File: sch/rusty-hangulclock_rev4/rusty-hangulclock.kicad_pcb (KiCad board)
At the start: 2 copper layers, 170 x 170 mm, 90 parts, among them J1 Conn_OLED, J2 Conn_OLED, J3 Conn_USB2, J4 USB_C_Receptacle_PowerOnly_6P, Q1 S8050, SW1 RotaryEncoder_Switch_MP, U1 ESP32-C3-WROOM-02, U2 SY8088, U3 DS3231MZ

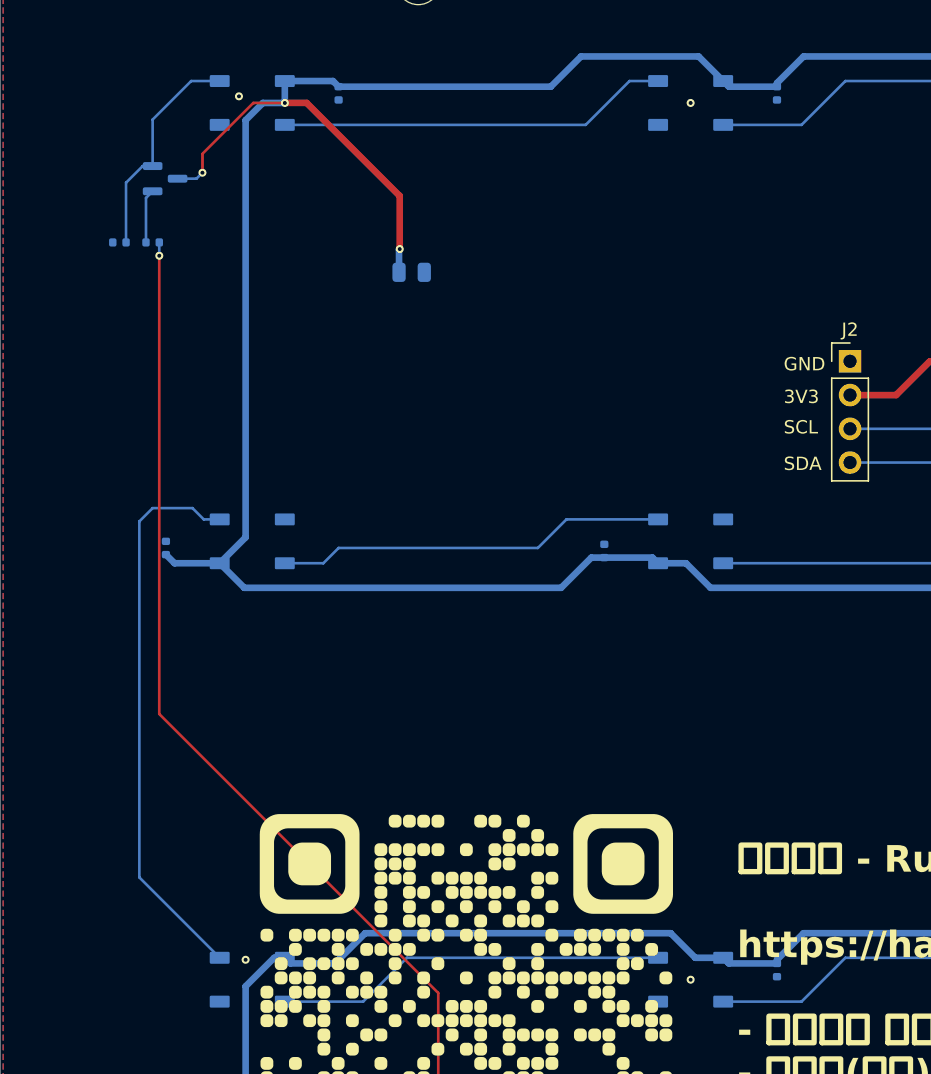
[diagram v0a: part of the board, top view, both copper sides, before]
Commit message: fix: sch
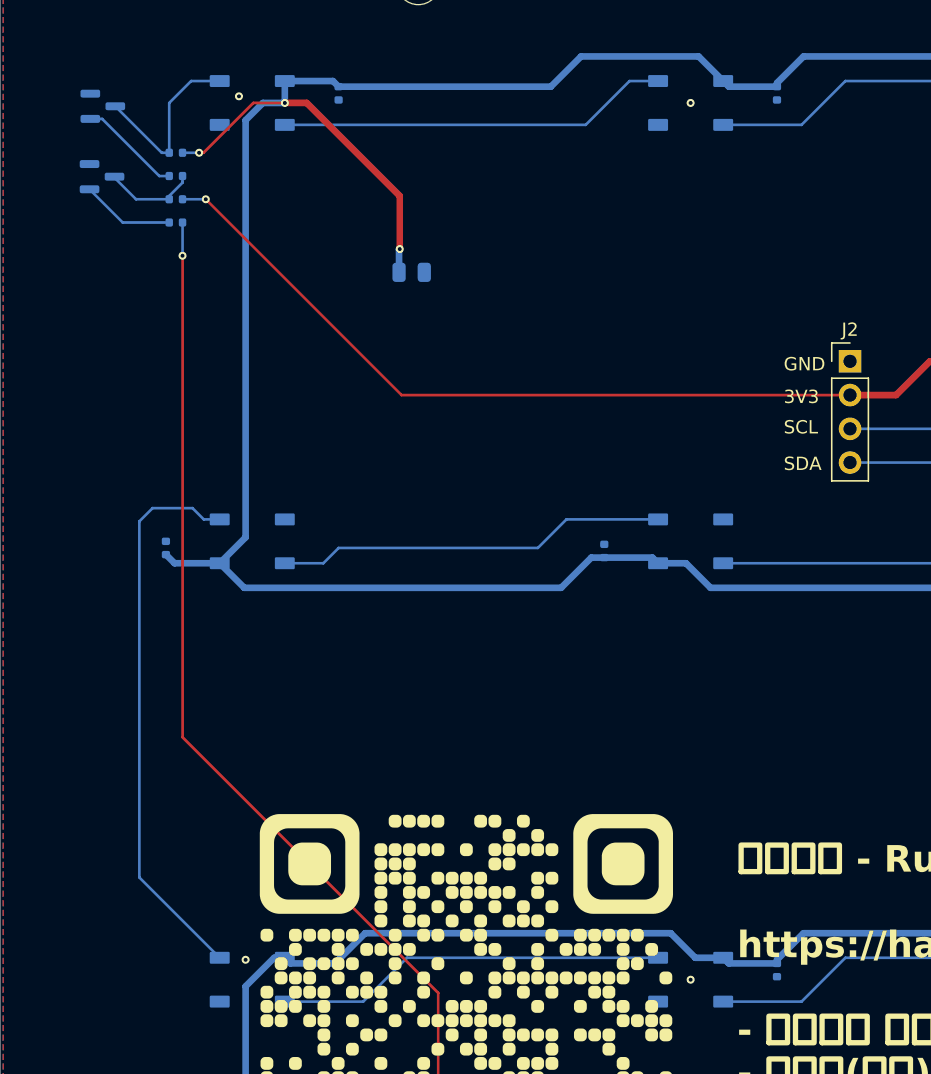
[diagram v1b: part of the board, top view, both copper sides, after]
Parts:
- removed R9: 10kΩ, PCM_JLCPCB:R_0402
- added Q2: S8050, PCM_JLCPCB:Q_SOT-23, B.Cu at (30.2, 41.8)
- added R10: 10kΩ, PCM_JLCPCB:R_0402, B.Cu at (35.8, 45.2)
- added R11: 10kΩ, PCM_JLCPCB:R_0402, B.Cu at (35.8, 48.8)
- added R5: 1kΩ, PCM_JLCPCB:R_0402, B.Cu at (35.8, 47.0)
- moved Q1 4.75 mm to (30.2, 47.0)
- moved R8 2.30 mm to (35.8, 50.5)
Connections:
- Q1 pad 2: LED_IN -> GND
- Q1 pad 3: +5V -> Net-(Q1-C)
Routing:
- net +3V3: track 249.4 -> 305.7 mm, vias 2 -> 3
- net Net-(Q2-B): track 0.00 -> 7.72 mm
- net Net-(Q1-C): track 0.00 -> 7.04 mm
- net LED_IN: track 17.1 -> 14.1 mm
- net Net-(Q1-B): track 4.06 -> 7.04 mm
- net +5V: track 968.2 -> 966.2 mm
- net IO6: track 164.1 -> 164.9 mm
